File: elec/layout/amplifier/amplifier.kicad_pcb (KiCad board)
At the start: 2 copper layers, 29 parts, among them U1 _Texas_Instruments_TAS5825MRH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

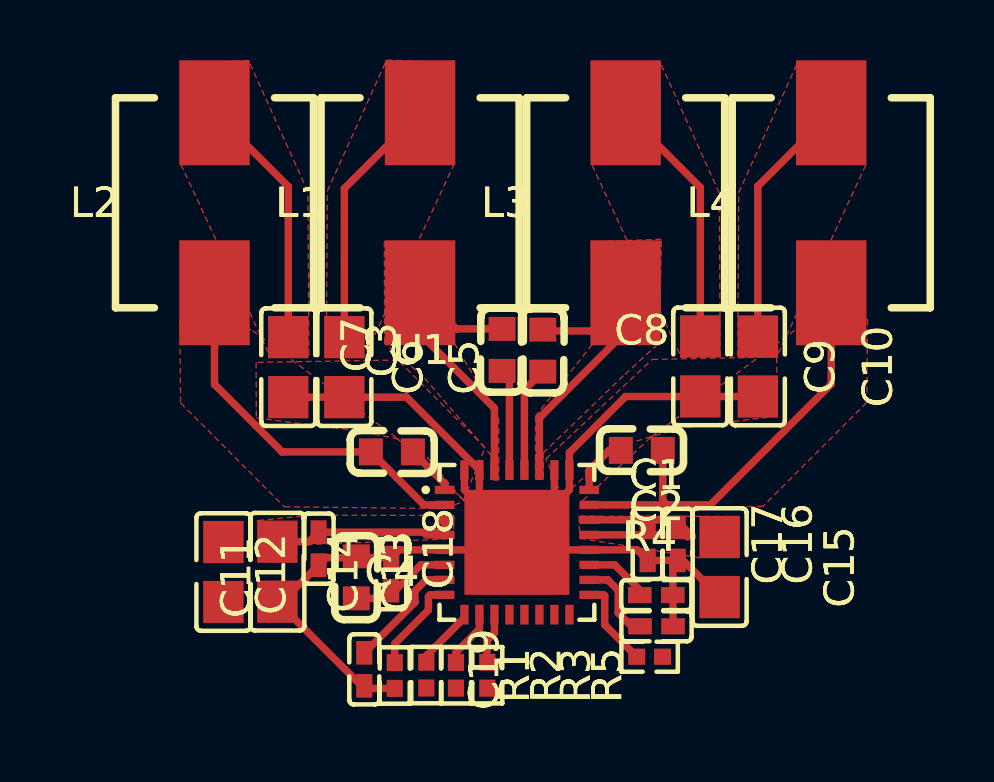
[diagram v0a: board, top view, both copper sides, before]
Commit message: Fix amplifier
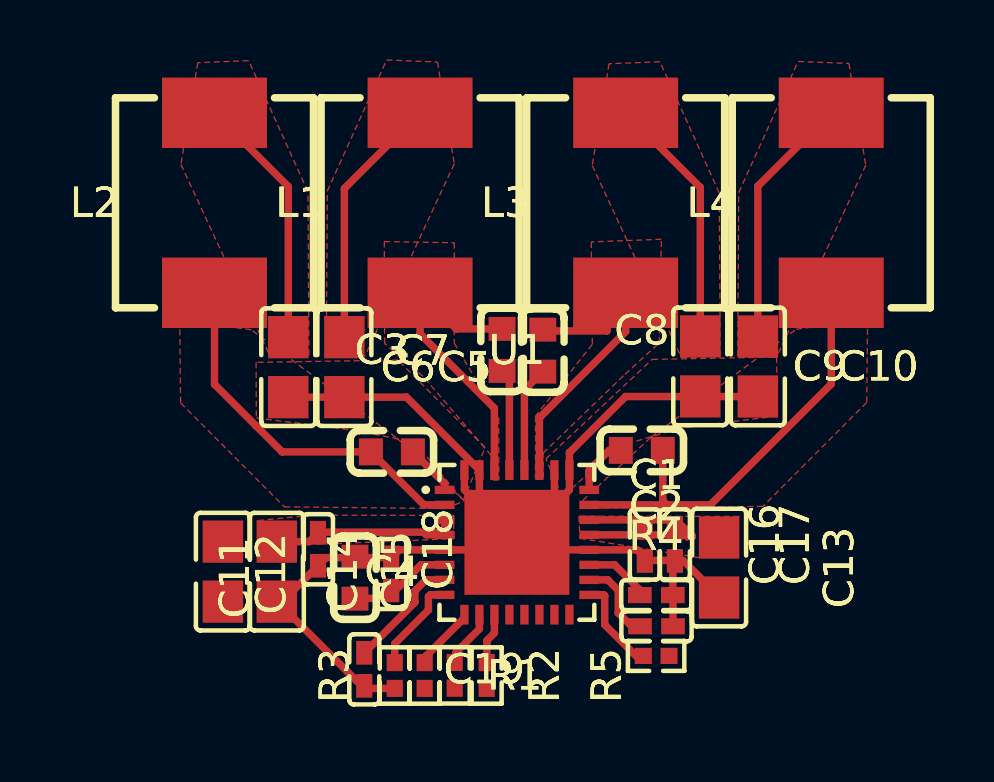
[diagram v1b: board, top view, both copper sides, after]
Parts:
- C1, C12, C16, C17, C18, C19, C2: footprint lcsc:C0402 -> atopile:C0402-b3ef17
- C10, C13, C14, C15, C5, C6, C9: footprint lcsc:C0805 -> atopile:C0805-3b2e55
- C11: value 4.7µF ±10% 16V X5R -> 4.7µF ±10% 10V X5R; footprint lcsc:C0603 -> atopile:C0603-bd72f6
- C3, C4, C7, C8: footprint lcsc:C0603 -> atopile:C0603-bd72f6
- L1, L2, L3, L4: value 10µH ±20% 4.5A 68mΩ -> (none); footprint lcsc:IND-SMD_L7.3-W6.8 -> atopile:IND-SMD_L7.3-W6.8-0bbdba
- R1, R2, R3, R4, R5: footprint lcsc:R0402 -> atopile:R0402-56259e
- U1: value _Texas_Instruments_TAS5825MRHBR -> (none); footprint lcsc:VQFN-32_L5.0-W5.0-P0.50-TL-EP -> atopile:VQFN-32_L5.0-W5.0-P0.50-TL-EP-7b5304
- moved C15 14.8 mm to (106.8, 115.6)
- moved C13 14.7 mm to (121.5, 115.4)
- moved C16 1.10 mm to (119.1, 114.7)
- moved C17 0.91 mm to (120.1, 114.7)
- moved R4 0.22 mm to (119.4, 118.4)
- moved R2 0.06 mm to (111.7, 119.0)
- turned R3 to 90 degrees
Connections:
- net fault-hv renamed hv-1
- net lrclk renamed LRCLK
- net mute-hv renamed hv-3
- net net renamed gnd
- net net-1 renamed BST_B_
- net net-10 renamed BST_A_
- net net-11 renamed BST_Bplus
- net net-12 renamed VR_DIG
- net net-13 renamed BST_Aplus
- net net-14 renamed OUT_Aplus
- net net-15 renamed GPIO0
- net net-16 renamed GPIO1
- net net-17 renamed PDNh
- net net-2 renamed OUT_B_
- net net-3 renamed ADR
- net net-4 renamed PVDD
- net net-5 renamed GVDD
- net net-6 renamed AVDD
- net net-7 renamed OUT_Bplus
- net net-8 renamed OUT_A_
- net net-9 renamed GPIO2
- net scl renamed SCL
- net sclk renamed SCLK
- net sda renamed SDA
- net sdin renamed SDIN
- net signal renamed line-3
- net signal-1 renamed line
- net signal-2 renamed line-1
- net signal-3 renamed line-2
- net warn-hv renamed hv-2
- C11 pad 1: hv -> DVDD
- C12 pad 1: hv -> DVDD
- R4 pad 2: pdn-hv -> hv
- U1 pad 6: hv -> DVDD
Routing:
- net hv: track 3.41 -> 0.00 mm
- net DVDD: track 0.00 -> 3.41 mm
- removed copper zone on F.Cu, net PVDD
